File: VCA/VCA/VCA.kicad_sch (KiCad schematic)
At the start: 54 parts, among them J1 VCO1, J2 VCO2, J3 VCO3, J4 VCO4, J5 Q1, J6 Q2, J7 Q3, J8 Q2, U1 SSI2164, U2 LM324

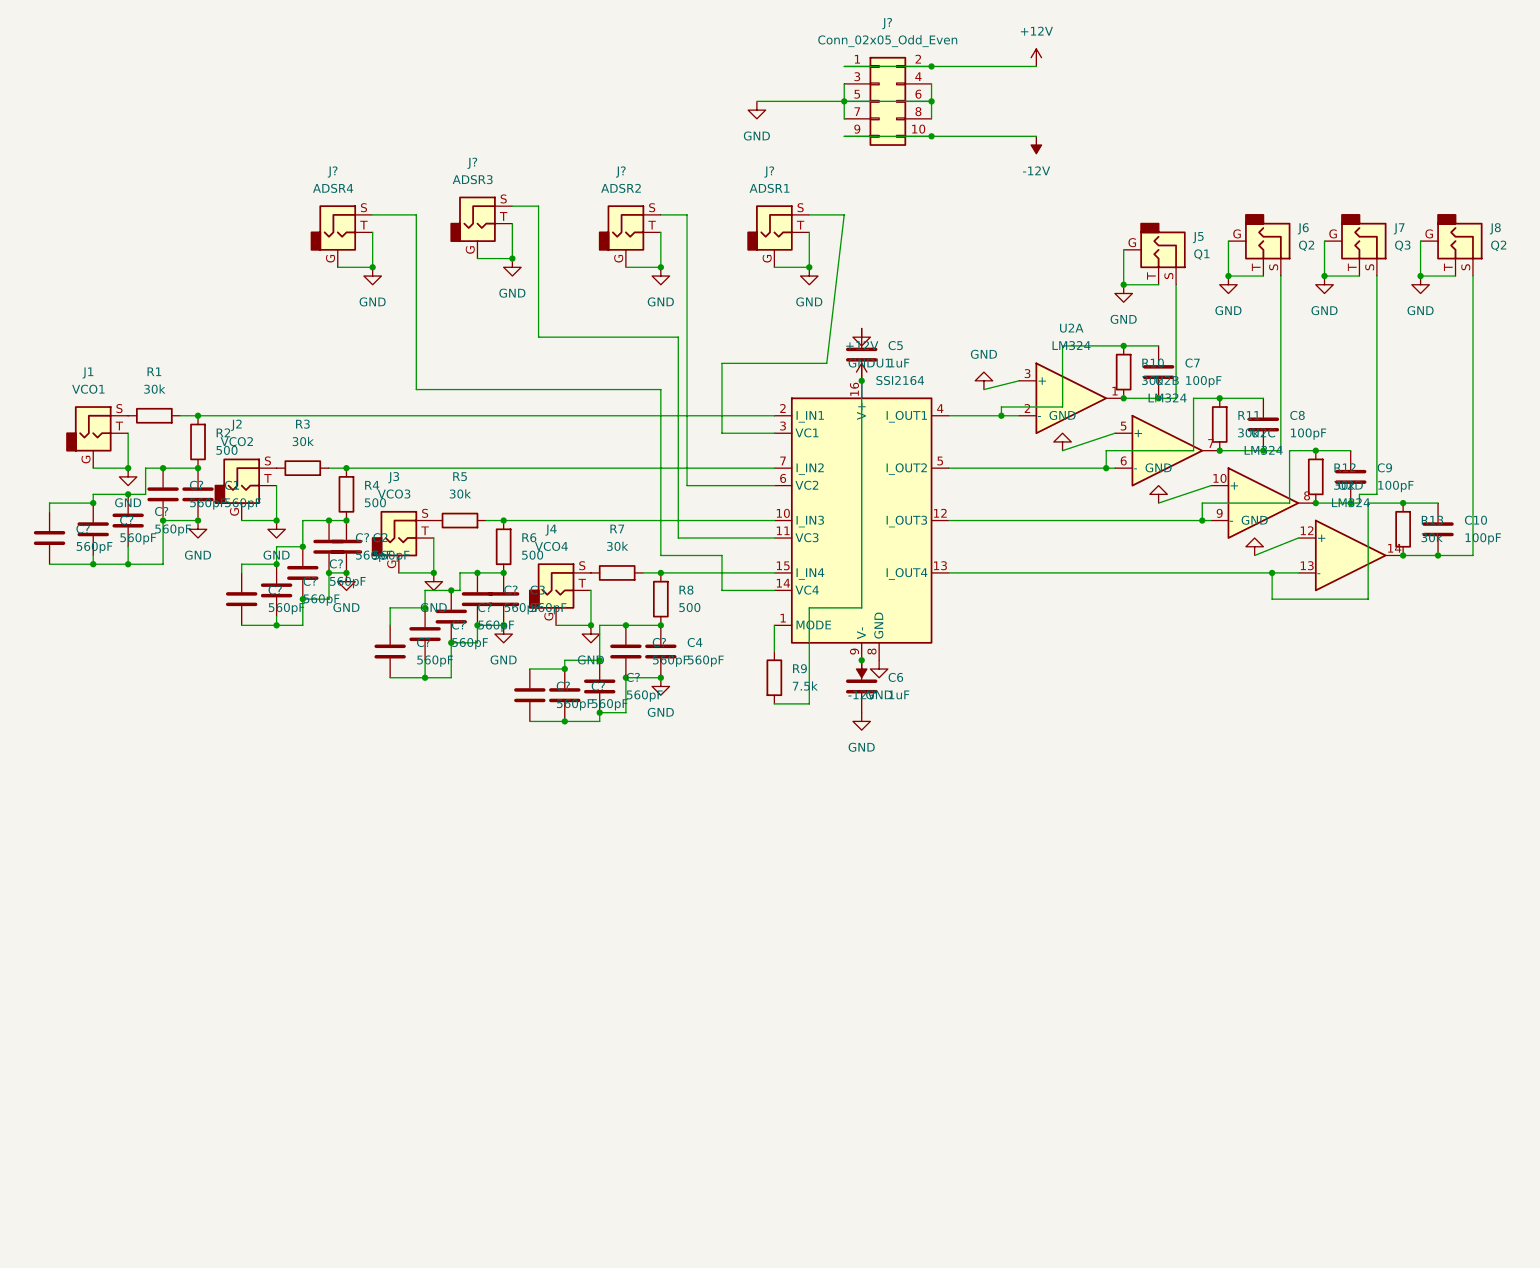
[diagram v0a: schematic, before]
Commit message: updated yo kengiz yawn guh bubby pirket
bubdaped yo dingdabing pep ring rong geeee renni
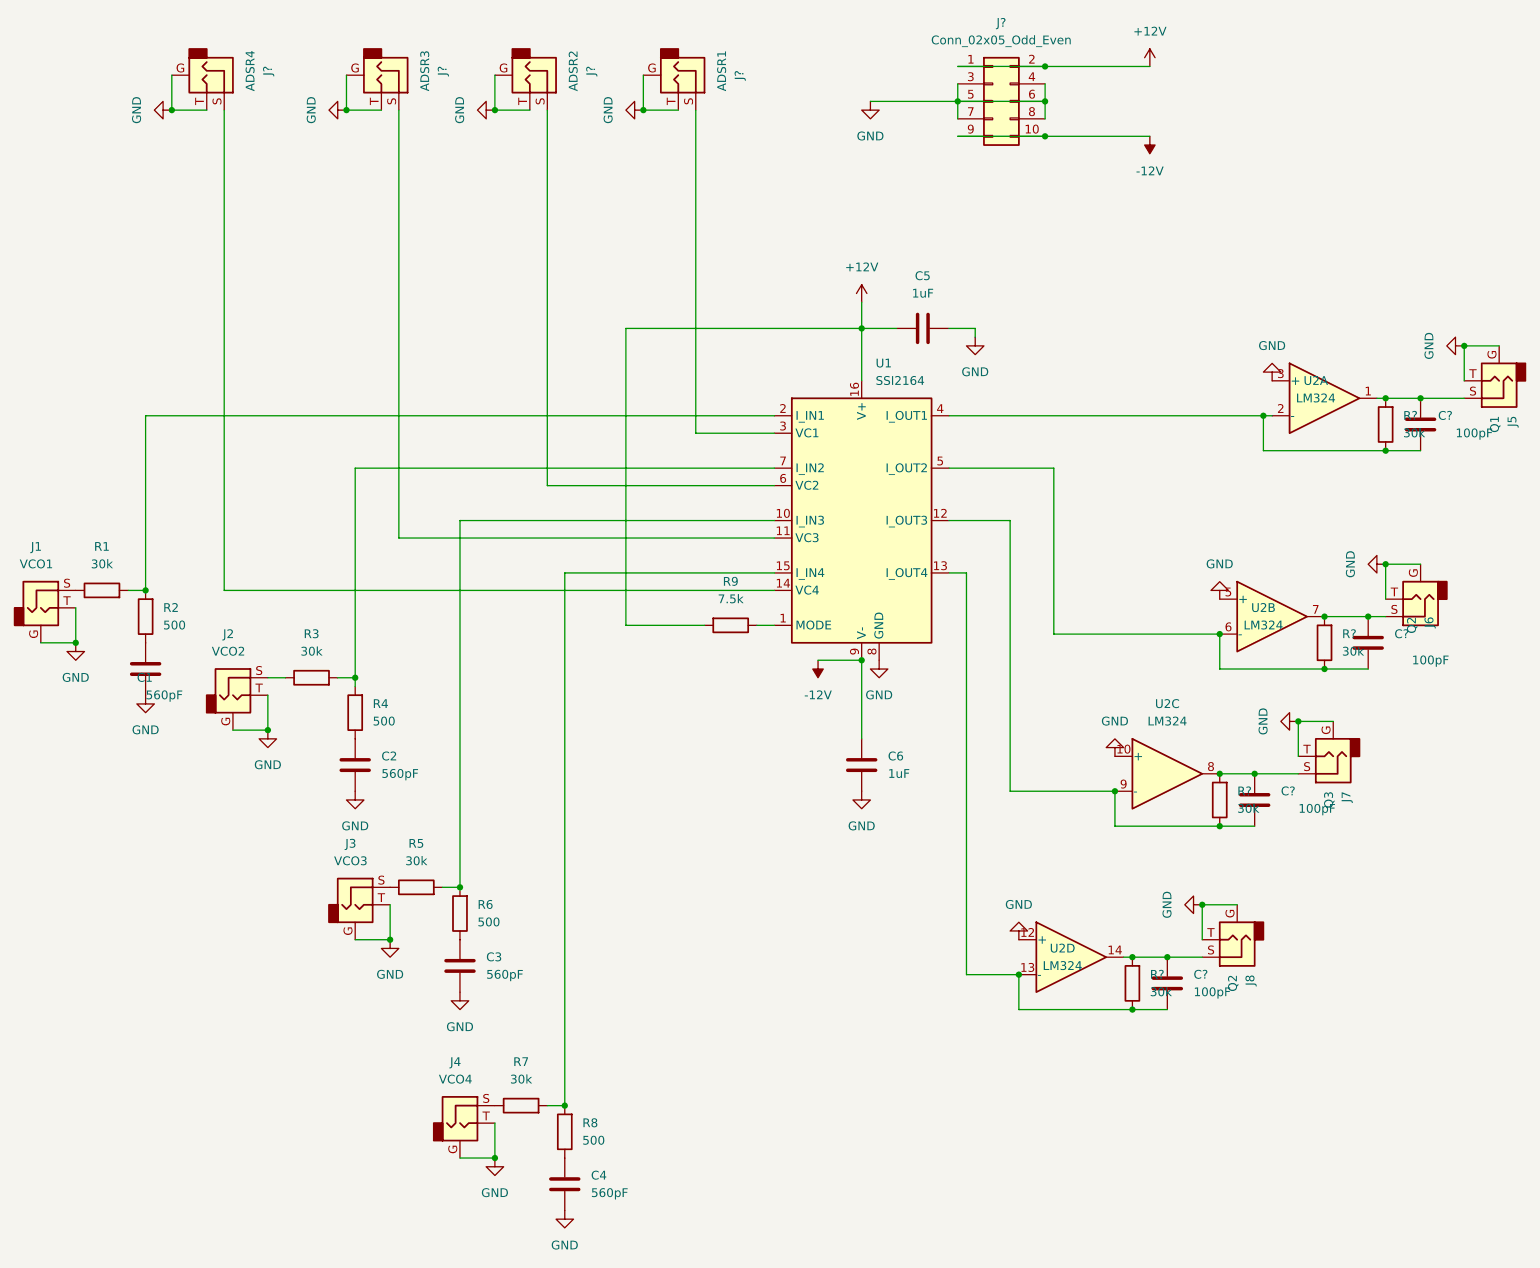
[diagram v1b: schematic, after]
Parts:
- removed C10, C7, C8, C9: 100pF, symbol Device:C
- removed C? (x16): 560pF, symbol Device:C
- removed R10, R11, R12, R13: 30k, symbol Device:R
- added C? (x4): 100pF, symbol Device:C
- added R? (x4): 30k, symbol Device:R
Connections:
- net at U1.5 (I_OUT2), U2.6 (-): now also C?.2, R?.1
- net at J6.S, U2.7: now also C?.1, R?.2
- net at J5.S, U2.1: now also C?.1, R?.2
- net at U1.4 (I_OUT1), U2.2 (-): now also C?.2, R?.1
- net at J7.S, U2.8: now also C?.1, R?.2
- net at U1.12 (I_OUT3), U2.9 (-): now also C?.2, R?.1
- net at J8.S, U2.14: now also C?.1, R?.2
- net at U1.13 (I_OUT4), U2.13 (-): now also C?.2, R?.1
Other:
- moved on the sheet: C1, C2, C3, C4, C5, C6, J1, J2, J3, J4, J5, J6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
